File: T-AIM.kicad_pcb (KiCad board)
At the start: 2 copper layers, 101.6 x 73.7 mm, 48 parts, among them IC1 ATMEGA328PB-A, IC2 MAX17043, J1 ADXL345 Connector, J2 PIR Sensor Connector, J3 JY-MCU HC-05 Pins, SW1 Connection Button, SW2 Reset Button, U1 TPS61200

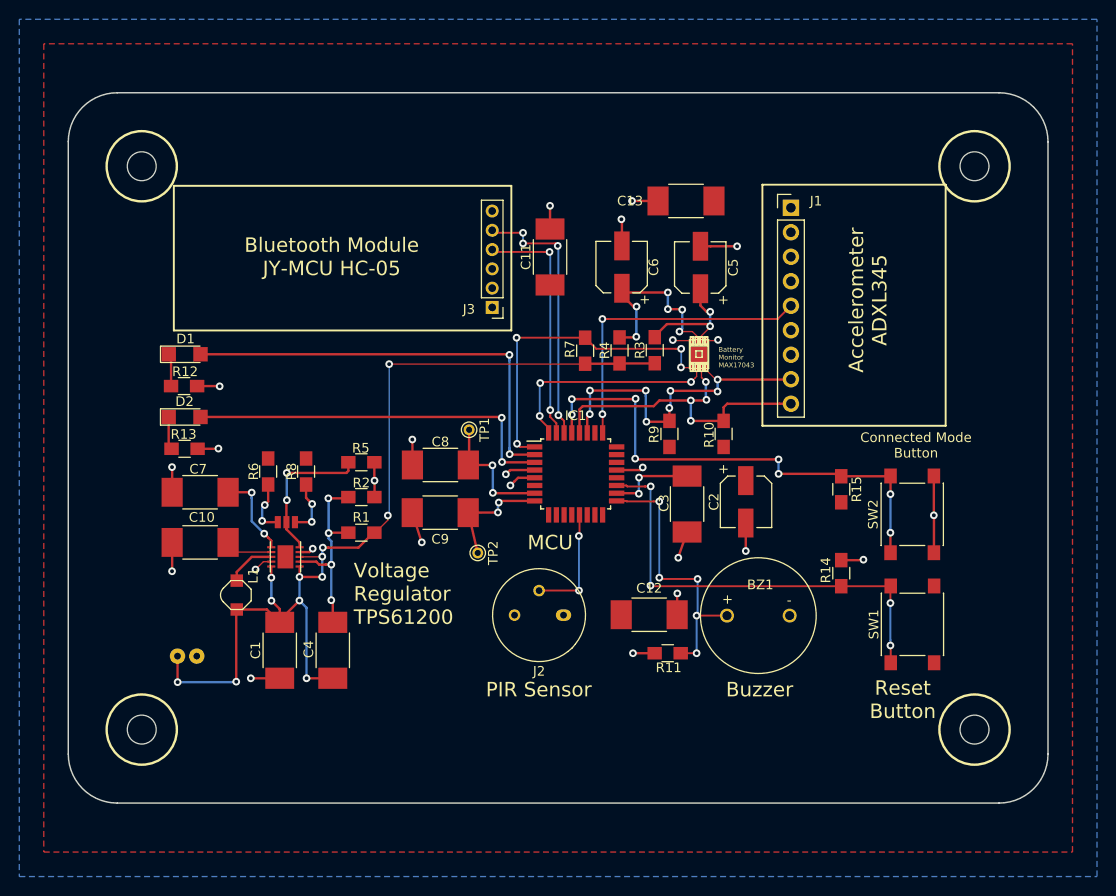
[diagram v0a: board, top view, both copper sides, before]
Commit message: PCB rebuilt
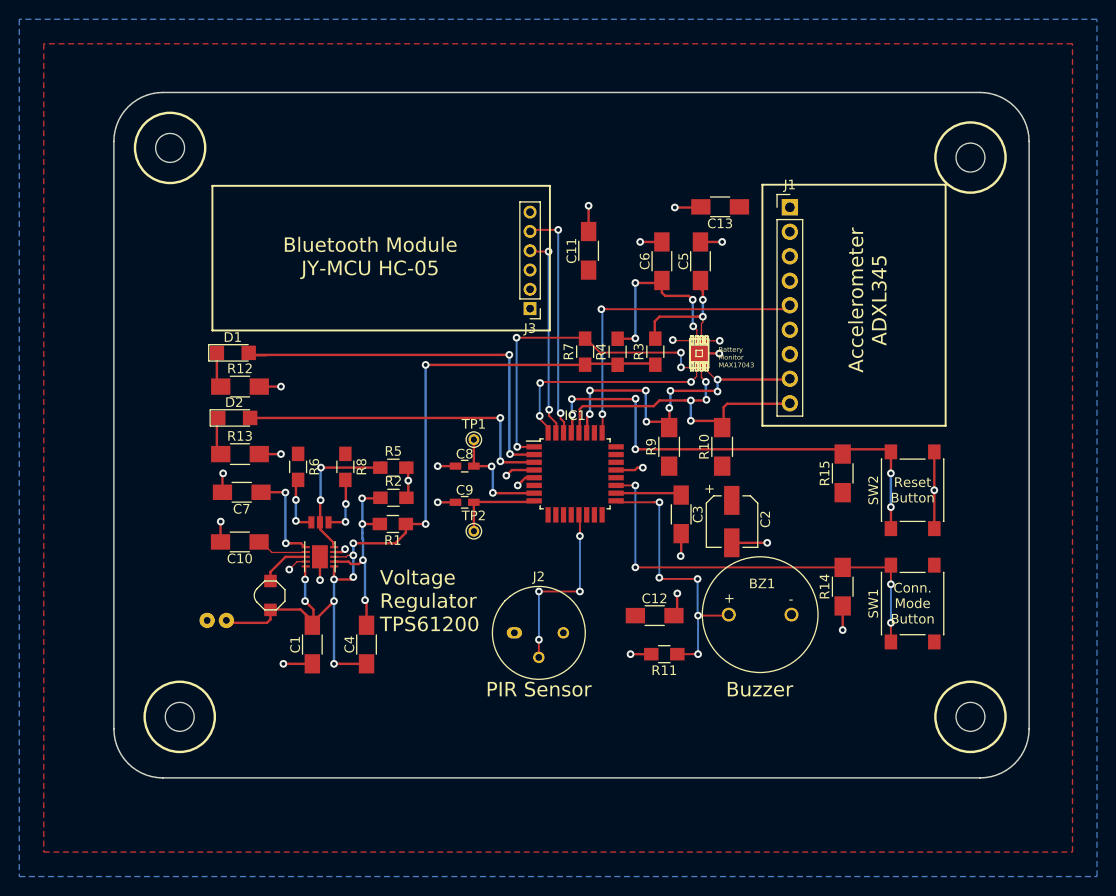
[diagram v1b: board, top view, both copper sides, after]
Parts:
- removed ? (x4): Screw_Hole_3_mm, T-AIM:Screw_Hole_3_mm
- added S**: Screw_Hole_3_mm, T-AIM:Screw_Hole_3_mm, F.Cu at (121.8, 59.3)
- added S**: Screw_Hole_3_mm, T-AIM:Screw_Hole_3_mm, F.Cu at (204.8, 60.3)
- added S**: Screw_Hole_3_mm, T-AIM:Screw_Hole_3_mm, F.Cu at (204.8, 118.3)
- added S**: Screw_Hole_3_mm, T-AIM:Screw_Hole_3_mm, F.Cu at (122.8, 118.3)
- C1, C10, C11, C12, C13, C3, C4, C7: footprint Capacitors_SMD:C_1812_HandSoldering -> Capacitors_SMD:C_1206_HandSoldering
- C5, C6: footprint Capacitors_SMD:CP_Elec_5x5.3 -> Capacitors_SMD:C_1206_HandSoldering
- C8, C9: footprint Capacitors_SMD:C_1812_HandSoldering -> Capacitors_SMD:C_0603_HandSoldering
- R10, R12, R13, R14, R15, R9: footprint Resistors_SMD:R_0805_HandSoldering -> Resistors_SMD:R_1206_HandSoldering
- SW2: value Reset Button -> Connection Button
- moved R12 5.80 mm to (129.1, 84.1)
- moved R13 5.78 mm to (129.1, 91.1)
- moved J2 5.42 mm to (157.5, 109.6), turned to 0 degrees
- moved D2 5.15 mm to (128.5, 87.3)
- moved D1 5.00 mm to (128.3, 80.6)
- moved JP1 4.81 mm to (126.7, 108.3), turned to 180 degrees
- moved C7 4.32 mm to (129.3, 95.1)
- moved C6 4.19 mm to (172.8, 71.1)
- moved C10 4.12 mm to (129.1, 100.2)
- moved R8 4.10 mm to (140.0, 92.4)
- moved C11 4.05 mm to (165.2, 70.0)
- moved J3 3.93 mm to (159.2, 76.0)
- moved C13 3.59 mm to (178.9, 65.5)
- moved U1 3.58 mm to (137.4, 101.7)
- moved C4 3.55 mm to (142.2, 110.8)
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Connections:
- R11 pad 1: GND -> AlarmBuzzer
- R11 pad 2: AlarmBuzzer -> GND
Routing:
- net VCC: track 108.2 -> 92.3 mm, vias 12 -> 10
- net PIR_OUT: track 12.0 -> 19.0 mm, vias 2 -> 4
- net GND: track 67.2 -> 61.1 mm
- net BlueLED: track 39.3 -> 34.2 mm
- net (no net): track 0.00 -> 4.52 mm, vias 0 -> 2
- net BL_TXD: track 25.1 -> 21.3 mm
- net RedLED: track 45.0 -> 41.6 mm
- net BL_RXD: track 27.8 -> 24.7 mm, vias 4 -> 2
- net Net-(C9-Pad1): track 12.2 -> 9.40 mm, vias 2 -> 0
- net ResetButton: track 52.5 -> 50.0 mm, vias 8 -> 6
- net 3V3: track 17.1 -> 14.9 mm, vias 3 -> 1
- net ConnectedButton: track 46.8 -> 45.1 mm
- net Net-(C6-Pad1): track 21.3 -> 19.6 mm, vias 6 -> 4
- net Net-(C8-Pad2): track 13.4 -> 11.7 mm
- net Net-(R5-Pad1): track 15.7 -> 16.4 mm
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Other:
- board size 101.6 x 73.7 mm -> 94.9 x 71.1 mm
- board text added: "Conn. Mode Button"
- board text removed: "Connected Mode Button"
- board text removed: "MCU"
